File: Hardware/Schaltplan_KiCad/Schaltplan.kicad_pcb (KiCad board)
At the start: 2 copper layers, 153 x 153 mm, 62 parts, among them IC1 LD1085V50, J1 3-106505-2, J2 USB_B_Micro, J3 Conn_01x04_Pin, J4 Conn_01x02_Pin, U1 MCP2562-E-SN, U2 FT231XS, U3 ESP32-DEVKITC-32U, U5 PCA9306DCTR

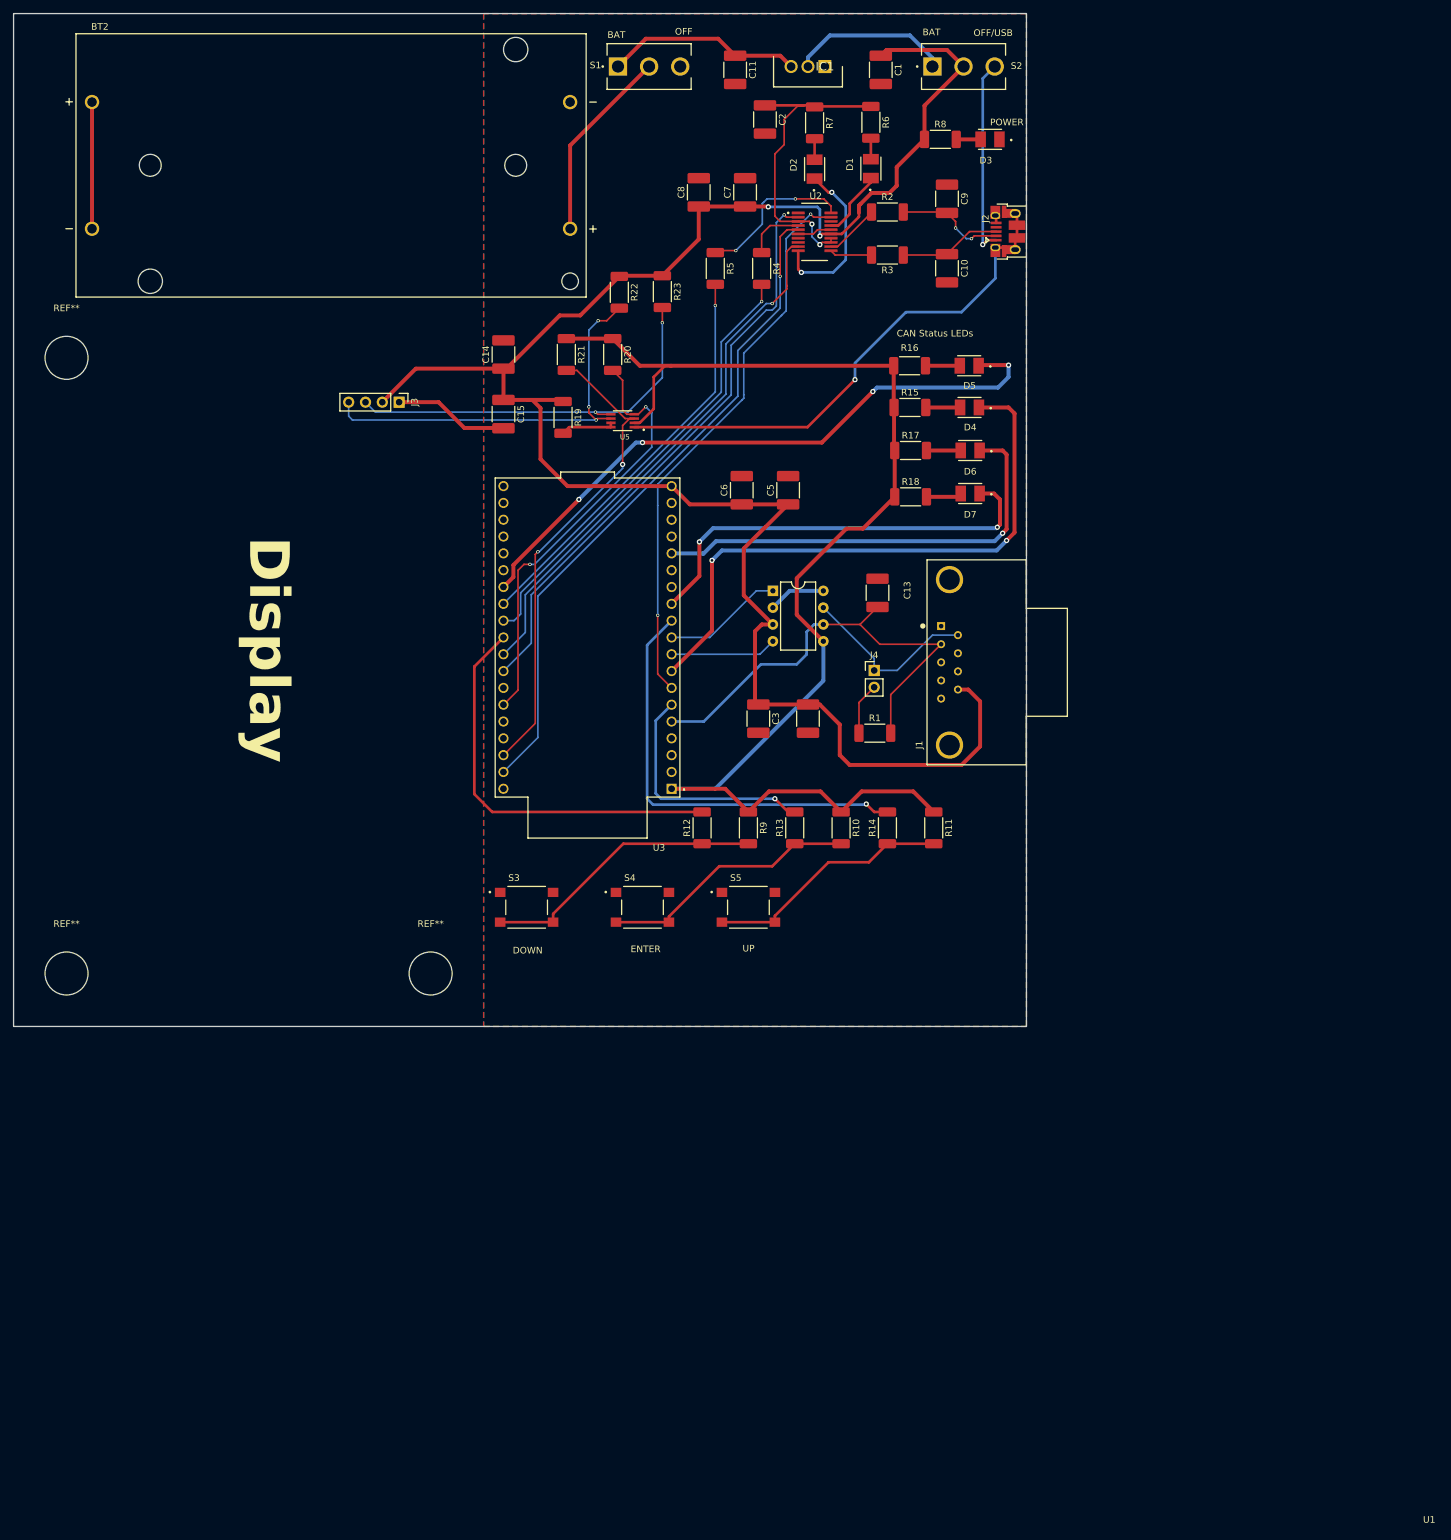
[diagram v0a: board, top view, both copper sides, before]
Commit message: finishes PCB Design
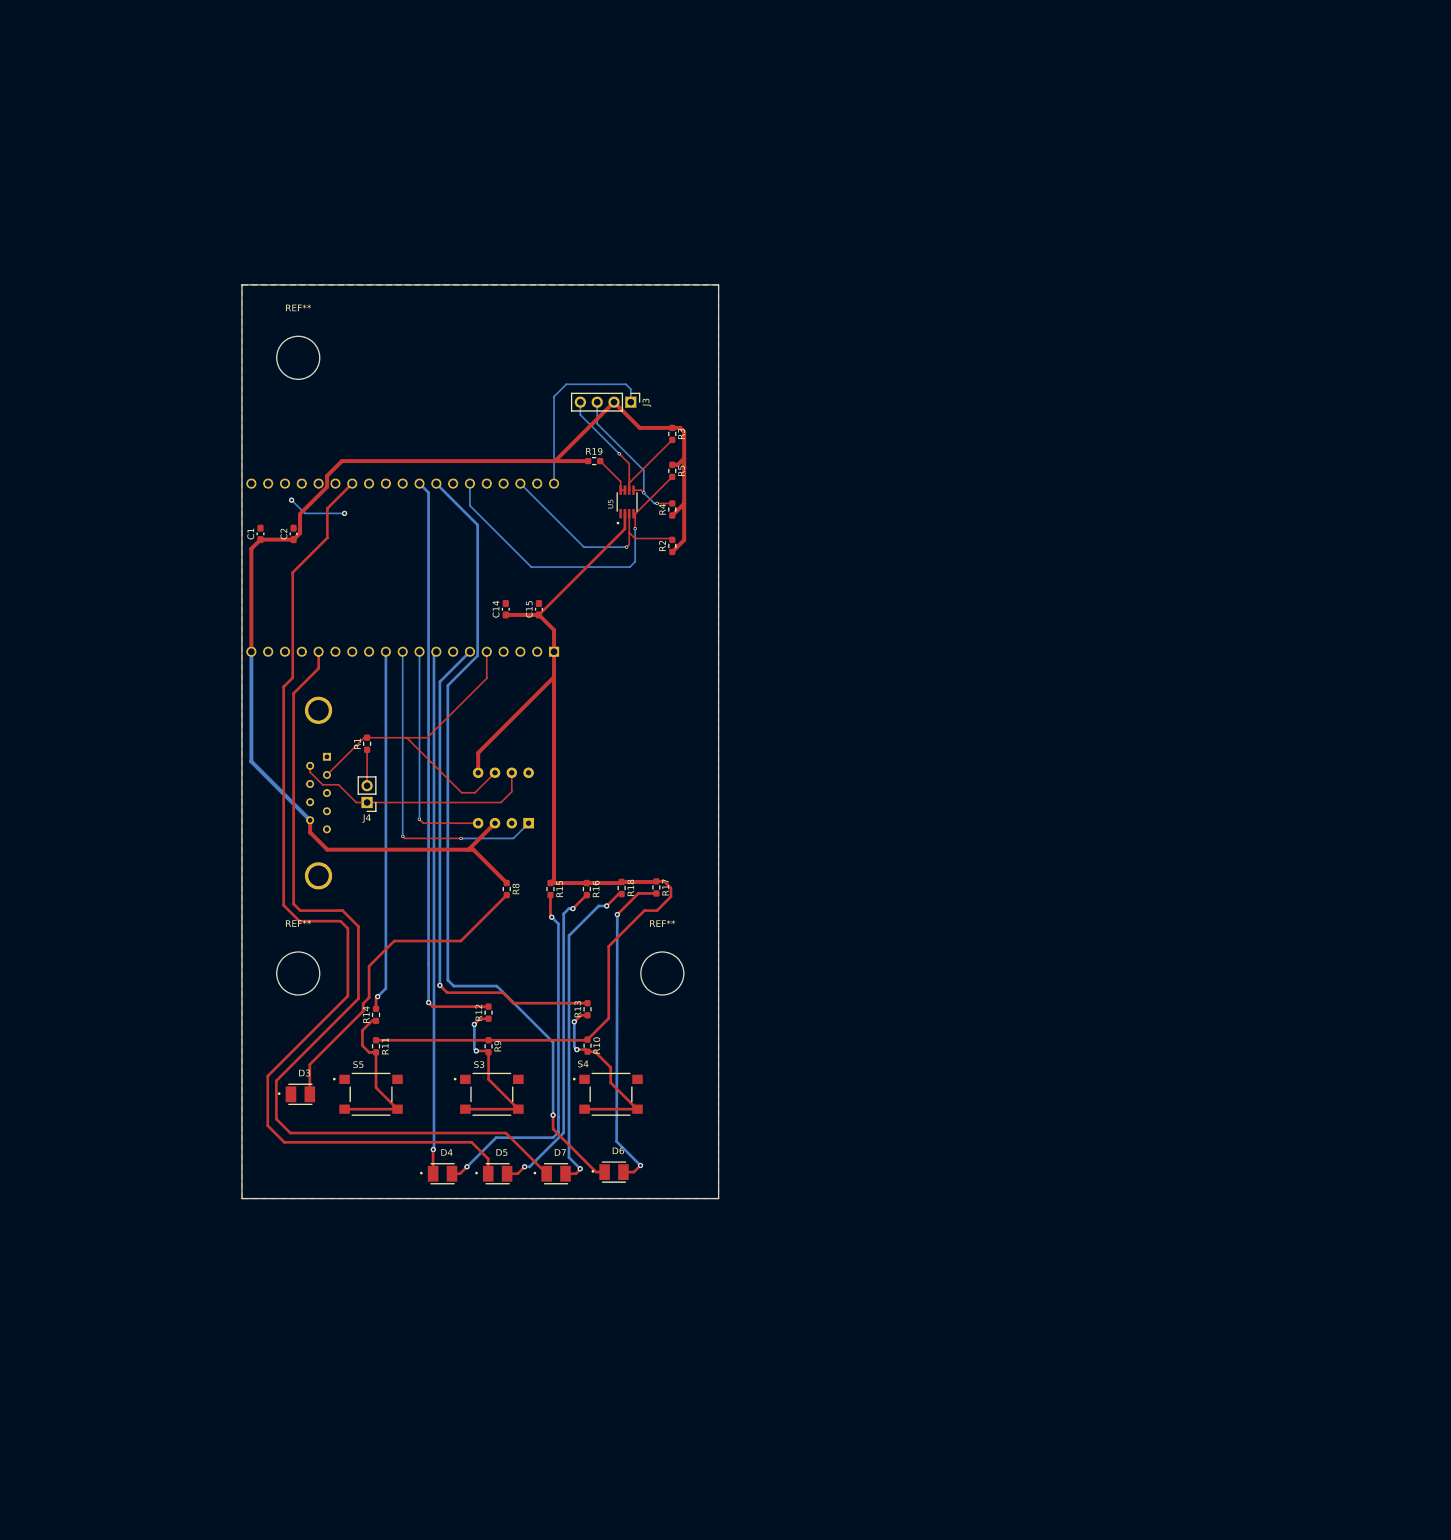
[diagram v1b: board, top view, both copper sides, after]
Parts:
- removed BT2: 1049, battery_holder:BAT_1049
- removed C10, C9: 47pF, Capacitor_SMD:C_1812_4532Metric_Pad1.57x3.40mm_HandSolder
- removed C11: 10uF, Capacitor_SMD:C_1812_4532Metric_Pad1.57x3.40mm_HandSolder
- removed C13: C, Capacitor_SMD:C_1812_4532Metric_Pad1.57x3.40mm_HandSolder
- removed C3, C5, C7: 100nF, Capacitor_SMD:C_1812_4532Metric_Pad1.57x3.40mm_HandSolder
- removed C4, C6, C8: 4.7uF, Capacitor_SMD:C_1812_4532Metric_Pad1.57x3.40mm_HandSolder
- removed D1, D2: LED, LED:LED_OF-SMD3528WC
- removed IC1: LD1085V50, LDO:TO255P460X1020X2008-3P
- removed J2: USB_B_Micro, Connector_USB:USB_Micro-B_Amphenol_10103594-0001LF_Horizontal
- removed R20, R21, R22, R23: 10k, Resistor_SMD:R_2010_5025Metric_Pad1.40x2.65mm_HandSolder
- removed R6, R7: 270, Resistor_SMD:R_2010_5025Metric_Pad1.40x2.65mm_HandSolder
- removed S1, S2: 1103M2S3CQE2, switches:SW_1103M2S3CQE2
- removed U2: FT231XS, USB2UART:SOP63P600X175-20N
- C1: value 22uF -> 100nF; footprint Capacitor_SMD:C_1812_4532Metric_Pad1.57x3.40mm_HandSolder -> Capacitor_SMD:C_0603_1608Metric_Pad1.08x0.95mm_HandSolder
- C14, C15: footprint Capacitor_SMD:C_1812_4532Metric_Pad1.57x3.40mm_HandSolder -> Capacitor_SMD:C_0603_1608Metric_Pad1.08x0.95mm_HandSolder
- C2: value C -> 4.7uF; footprint Capacitor_SMD:C_1812_4532Metric_Pad1.57x3.40mm_HandSolder -> Capacitor_SMD:C_0603_1608Metric_Pad1.08x0.95mm_HandSolder
- J1, U1, U3: moved to B.Cu
- R1: value R -> 120R; footprint Resistor_SMD:R_2010_5025Metric_Pad1.40x2.65mm_HandSolder -> Resistor_SMD:R_0603_1608Metric_Pad0.98x0.95mm_HandSolder
- R10, R11, R12, R13, R14, R15, R16, R17, R18, R19, R8, R9: footprint Resistor_SMD:R_2010_5025Metric_Pad1.40x2.65mm_HandSolder -> Resistor_SMD:R_0603_1608Metric_Pad0.98x0.95mm_HandSolder
- R2, R3: value 27R -> 10k; footprint Resistor_SMD:R_2010_5025Metric_Pad1.40x2.65mm_HandSolder -> Resistor_SMD:R_0603_1608Metric_Pad0.98x0.95mm_HandSolder
- R4, R5: value R -> 10k; footprint Resistor_SMD:R_2010_5025Metric_Pad1.40x2.65mm_HandSolder -> Resistor_SMD:R_0603_1608Metric_Pad0.98x0.95mm_HandSolder
- moved D3 177.9 mm to (56.3, 178.2), turned to 0 degrees
- moved D5 141.3 mm to (86.1, 190.2), turned to 0 degrees
- moved D4 140.5 mm to (77.8, 190.2), turned to 0 degrees
- moved R8 130.8 mm to (87.5, 147.2), turned to -90 degrees
- moved D6 121.6 mm to (103.7, 190.0), turned to 0 degrees
- moved D7 120.3 mm to (95.0, 190.2), turned to 0 degrees
- moved C1 117.0 mm to (50.3, 93.6), turned to 90 degrees
- moved J1 94.9 mm to (60.3, 127.3)
- moved C2 94.8 mm to (55.3, 93.6), turned to 90 degrees
- moved R16 92.9 mm to (99.6, 147.2), turned to -90 degrees
- moved R15 90.8 mm to (94.1, 147.2), turned to -90 degrees
- moved R11 90.5 mm to (67.8, 171.0)
- moved R14 82.3 mm to (67.8, 166.2)
- moved J4 79.2 mm to (66.4, 134.2), turned to 180 degrees
- moved R1 76.7 mm to (66.4, 125.3), turned to 90 degrees
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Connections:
- C14 pad 1: +5V -> +3V3
- C15 pad 1: +5V -> +3V3
- C2 pad 1: /FT231_3V3_OUT -> +5V
- D6 pad 1: /ESP32_IO13 -> /ESP32_IO19
- D7 pad 1: /ESP32_IO14 -> /ESP32_IO13
- R12 pad 2: /ESP32_IO5 -> /ESP32_IO18
- R2 pad 1: /FT231_USBDM -> +5V
- R2 pad 2: /USBDM -> /ESP32_SCL1
- R3 pad 1: /USBDP -> +5V
- R3 pad 2: /FT231_USBDP -> /DISPLAY_SCL2
- R4 pad 1: /FT231_RX -> +5V
- R4 pad 2: /ESP32TX -> /DISPLAY_SDA2
- R5 pad 1: /FT231_TX -> +5V
- R5 pad 2: /ESP32RX -> /ESP32_SDA1
- U3 pad 12: /ESP32_IO14 -> unconnected-(U3-IO14-Pad12)
- U3 pad 27: /ESP32RX -> unconnected-(U3-IO16-Pad27)
- U3 pad 28: /ESP32TX -> unconnected-(U3-IO17-Pad28)
- U3 pad 29: /ESP32_IO5 -> unconnected-(U3-IO5-Pad29)
- U3 pad 30: /FT231_CTS -> /ESP32_IO18
- U3 pad 31: /FT231_RTS -> /ESP32_IO19
- U3 pad 37: /FT231_RI -> unconnected-(U3-IO23-Pad37)
- U3 pad 7: /FT231_SLEEP -> unconnected-(U3-IO32-Pad7)
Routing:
- net /ESP32_IO19: track 0.00 -> 122.8 mm, vias 0 -> 1
- net /FT231_RI: track 101.3 -> 0.00 mm, vias 1 -> 0
- net +5V: track 290.2 -> 192.7 mm, vias 2 -> 0
- net /FT231_RTS: track 89.3 -> 0.00 mm, vias 1 -> 0
- net /ESP32_IO18: track 0.00 -> 88.3 mm, vias 0 -> 1
- net /FT231_SLEEP: track 85.3 -> 0.00 mm, vias 2 -> 0
- net /FT231_CTS: track 81.1 -> 0.00 mm, vias 1 -> 0
- net GNDREF: track 111.6 -> 36.6 mm, vias 1 -> 2
- net /ESP32TX: track 67.9 -> 0.00 mm, vias 1 -> 0
- net /ESP32_IO14: track 64.8 -> 0.00 mm, vias 2 -> 0
- net /ESP32_IO13: track 67.8 -> 129.4 mm, vias 1 -> 0
- net /ESP32RX: track 61.5 -> 0.00 mm, vias 1 -> 0
- net /ESP32_IO5: track 61.0 -> 0.00 mm
- net /ESP32_IO4: track 96.9 -> 151.6 mm, vias 4 -> 0
- net Net-(D4-A): track 5.17 -> 55.0 mm, vias 0 -> 2
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- removed copper zone on B.Cu, net GNDREF
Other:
- board size 153 x 153 mm -> 72 x 138 mm
- board text removed: "BAT"
- board text removed: "CAN Status LEDs"
- board text removed: "DOWN"
- board text removed: "Display"
- board text removed: "ENTER"
- board text removed: "OFF"
- board text removed: "OFF/USB"
- board text removed: "POWER"
- board text removed: "UP"
